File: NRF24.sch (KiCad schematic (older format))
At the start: 43 parts, among them J1 Conn_ARM_JTAG_SWD_10, J2 SMA, Q1 NTK3139P, Q2 NTK3139P, U1 Si7021-A20, U2 STM32L031G6Ux, U3 nRF24L01P, Y1 16MHz

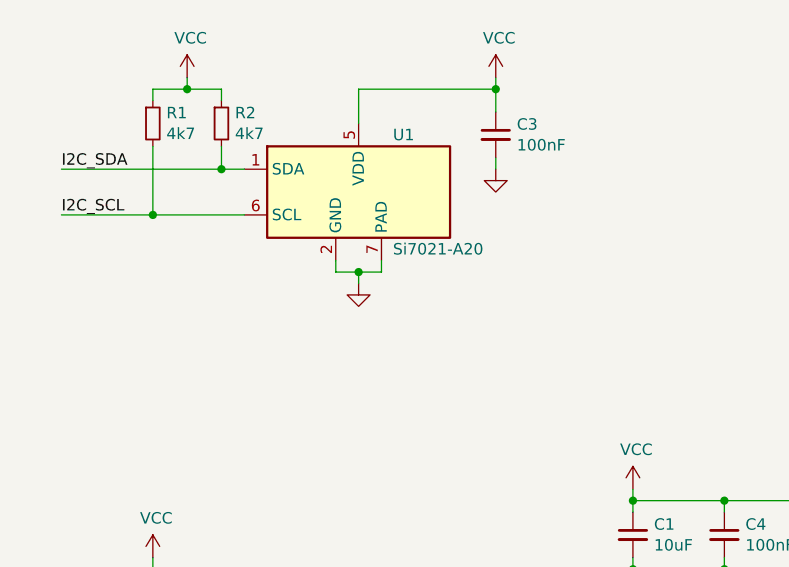
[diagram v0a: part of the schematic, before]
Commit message: Layout
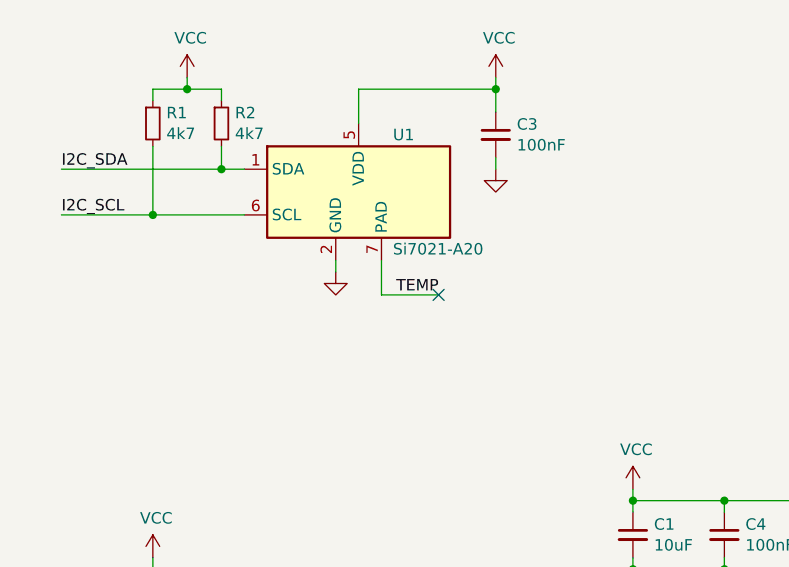
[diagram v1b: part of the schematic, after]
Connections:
- net GND: no longer U1.7 (PAD)
- new net TEMP: U1.7 (PAD)
- no-connect marks 10 -> 11
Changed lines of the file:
@@
 L power:GND #PWR06
 U 1 1 5F6F7763
-P 2300 3250
-F 0 "#PWR06" H 2300 3000 50  0001 C CNN
-F 1 "GND" H 2305 3077 50  0001 C CNN
-F 2 "" H 2300 3250 50  0001 C CNN
-F 3 "" H 2300 3250 50  0001 C CNN
-	1    2300 3250
+P 2200 3200
+F 0 "#PWR06" H 2200 2950 50  0001 C CNN
+F 1 "GND" H 2205 3027 50  0001 C CNN
+F 2 "" H 2200 3200 50  0001 C CNN
+F 3 "" H 2200 3200 50  0001 C CNN
+	1    2200 3200
 	1    0    0    -1
 $EndComp
@@
 Wire Wire Line
 	2900 2400 2900 2500
-Wire Wire Line
-	2200 3150 2200 3200
-Wire Wire Line
-	2200 3200 2300 3200
-Wire Wire Line
-	2400 3200 2400 3150
-Wire Wire Line
-	2300 3250 2300 3200
-Connection ~ 2300 3200
-Wire Wire Line
-	2300 3200 2400 3200
 Wire Wire Line
 	1350 5800 1350 5750
@@
 	1    0    0    -1
 $EndComp
+Wire Wire Line
+	2200 3150 2200 3200
+Wire Wire Line
+	2400 3300 2650 3300
+Wire Wire Line
+	2400 3150 2400 3300
+Text Label 2650 3300 2    50   ~ 0
+TEMP
+NoConn ~ 2650 3300
 $EndSCHEMATC
